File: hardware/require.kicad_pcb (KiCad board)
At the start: 6 copper layers, 70 x 25.4 mm, 99 parts, among them J1 Conn_01x02, U100 SY8089AAC, U1000 RK3308, U15 SY8088AAC, U200 SY8089AAC, U3 EMMC_BGA_153, U300 SY8089AAC, U3000 DDR3_FBGA96, U6000 ap6255, Y1 Crystal_GND24

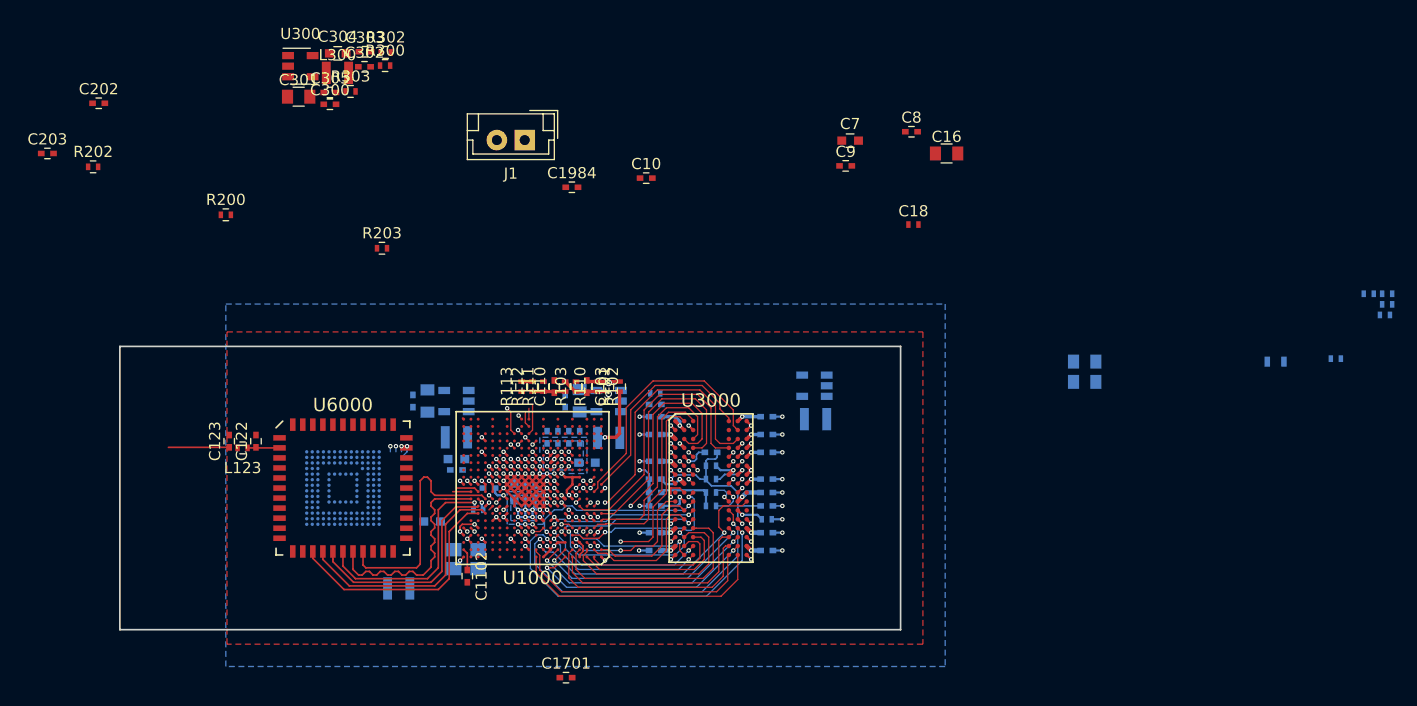
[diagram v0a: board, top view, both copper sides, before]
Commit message: wip
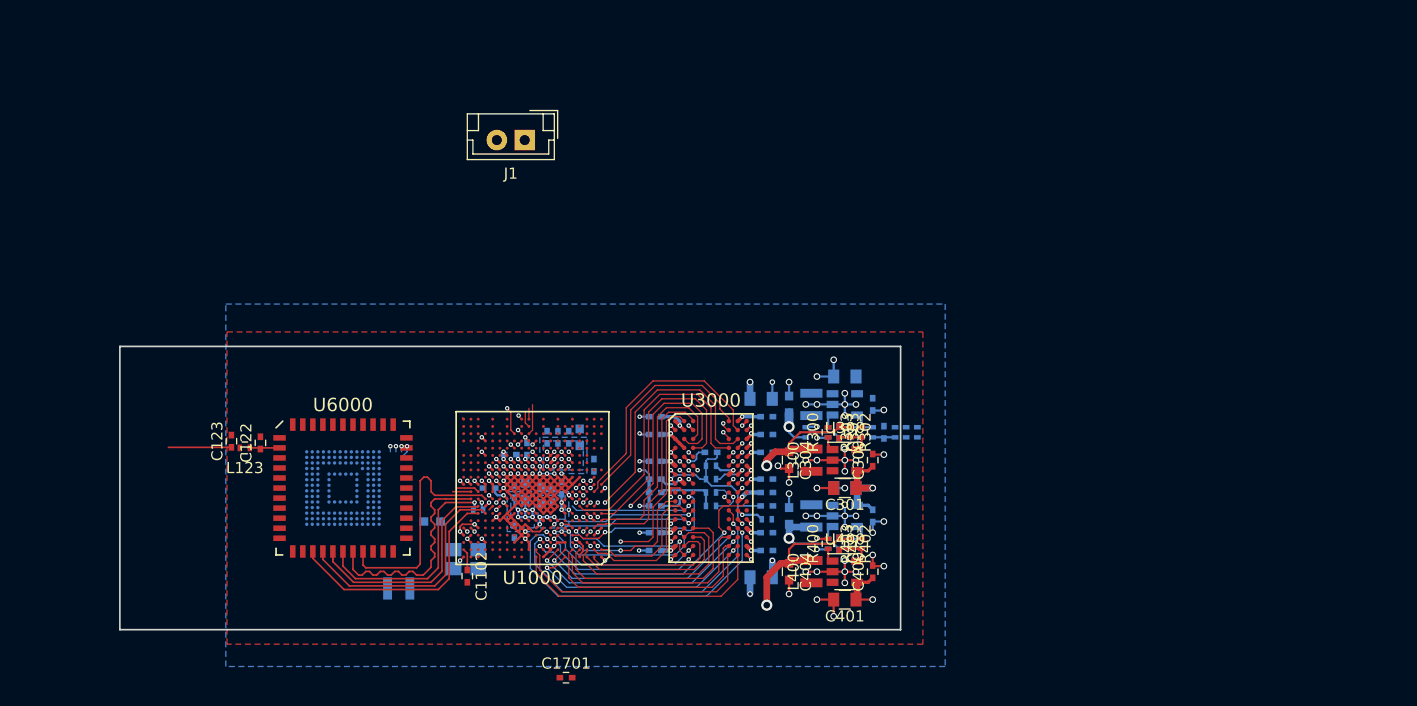
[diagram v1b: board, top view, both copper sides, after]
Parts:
- removed C10: C, Capacitors_SMD:C_0402
- removed C102, C202, C302: 1n, Capacitors_SMD:C_0402
- removed C16: 10uF,10V,X5R, Capacitors_SMD:C_0805
- removed C18: 1u, Resistors_SMD:R_0402_NoSilk
- removed C20: 22p, Resistors_SMD:R_0402_NoSilk
- removed C205, C305: 0.1u, Capacitors_SMD:C_0402
- removed C22: 22u, Resistors_SMD:R_0603
- removed C24: 0.1u, Resistors_SMD:R_0402_NoSilk
- removed L3: 3.3u, require:L_murata_2520
- removed R10: 10, Resistors_SMD:R_0402_NoSilk
- removed R7: 10k, Resistors_SMD:R_0402_NoSilk
- removed R9: 100,5%, Resistors_SMD:R_0402_NoSilk
- removed U15: SY8088AAC, TO_SOT_Packages_SMD:SOT-23-5
- added C400: 0.1u,10V, Capacitors_SMD:C_0402, F.Cu at (95.5, 72.5)
- added C401: 10u,10V, Capacitors_SMD:C_0805, F.Cu at (93.0, 75.0)
- added C403: 22p, Capacitors_SMD:C_0402, F.Cu at (92.5, 70.0)
- added C404: 22u, Capacitors_SMD:C_0603, F.Cu at (88.0, 72.5)
- added C5123: 0.1u, Capacitors_SMD:C_0402, B.Cu at (64.5, 61.5)
- added C5124: 0.1u, Capacitors_SMD:C_0402, B.Cu at (70.5, 63.0)
- added L400: 2.2u, require:L_murata_2520, F.Cu at (90.0, 72.5)
- added R400: 10k, Resistors_SMD:R_0402, F.Cu at (91.5, 70.0)
- added R402: 110k,1%, Resistors_SMD:R_0402, F.Cu at (93.5, 70.0)
- added R403: 150k,1%, Resistors_SMD:R_0402, F.Cu at (94.5, 70.0)
- added U400: SY8089AAC, TO_SOT_Packages_SMD:SOT-23-5, F.Cu at (93.0, 72.5)
- C103, C110, C1984, C203, R101, R102, R103, R110, R111, R112, R113, R200, R202, R203: moved to B.Cu
- C107: value 0.1u -> 2.2u
- C108: value 0.1u -> 22u; footprint Capacitors_SMD:C_0402 -> Capacitors_SMD:C_0603
- C310: renamed from C7; value C -> 10u; moved to B.Cu
- C311: renamed from C8; value C -> 0.1u; moved to B.Cu
- C312: renamed from C9; value C -> 0.1u; moved to B.Cu
- moved C203 79.2 mm to (92.5, 70.0), turned to 90 degrees
- moved R202 75.8 mm to (93.5, 70.0), turned to 90 degrees
- moved R200 61.5 mm to (91.5, 70.0), turned to 270 degrees
- moved U300 60.3 mm to (93.0, 62.5)
- moved C301 60.2 mm to (93.0, 65.0), turned to 180 degrees
- moved C300 58.2 mm to (95.5, 62.5), turned to 90 degrees
- moved R303 55.1 mm to (94.5, 60.0), turned to 90 degrees
- moved L300 54.9 mm to (90.0, 62.5), turned to 90 degrees
- moved C303 54.5 mm to (92.5, 60.0), turned to 270 degrees
- moved C304 54.5 mm to (88.0, 62.5), turned to 270 degrees
- moved R302 53.8 mm to (93.5, 60.0), turned to 270 degrees
- moved R300 51.6 mm to (91.5, 60.0), turned to 90 degrees
- moved R203 50.5 mm to (94.5, 70.0), turned to 270 degrees
- moved C311 45.8 mm to (66.8, 65.7), turned to 90 degrees
- moved C200 42.5 mm to (95.5, 67.5), turned to 270 degrees
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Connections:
- C303 pad 1: VDD_CORE -> VCC_DDR
- C304 pad 1: VDD_CORE -> VCC_DDR
- L300 pad 2: VDD_CORE -> VCC_DDR
- R302 pad 1: VDD_CORE -> VCC_DDR
- U1000 pad G15: Net-(U1000-PadG15) -> GND
- U1000 pad N2: (no net) -> Net-(U1000-PadN2)
- U1000 pad N3: (no net) -> /rk3308-lcdc-mac-i2s1-jtag/WIFI_WAKE_HOST
- U1000 pad N4: (no net) -> Net-(U1000-PadN4)
- U1000 pad N5: (no net) -> VCC_IO
- U1000 pad P3: (no net) -> /rk3308-lcdc-mac-i2s1-jtag/WIFI_REG_ON
- U1000 pad P4: (no net) -> Net-(U1000-PadP4)
- U1000 pad R11: (no net) -> VCC_IO
- U1000 pad R3: (no net) -> Net-(U1000-PadR3)
- U1000 pad R4: (no net) -> Net-(U1000-PadR4)
- U1000 pad R9: (no net) -> Net-(U1000-PadR9)
- U1000 pad T1: (no net) -> Net-(U1000-PadT1)
- U1000 pad T10: (no net) -> /rk3308-lcdc-mac-i2s1-jtag/SPI2_CS
- U1000 pad T2: (no net) -> Net-(U1000-PadT2)
- U1000 pad T3: (no net) -> Net-(U1000-PadT3)
- U1000 pad T4: (no net) -> Net-(U1000-PadT4)
- U1000 pad T5: (no net) -> Net-(U1000-PadT5)
- U1000 pad T6: (no net) -> Net-(U1000-PadT6)
- U1000 pad T8: (no net) -> Net-(U1000-PadT8)
- U1000 pad T9: (no net) -> /rk3308-lcdc-mac-i2s1-jtag/SPI2_TX_UART2_TX_M0
- U1000 pad U2: (no net) -> Net-(U1000-PadU2)
- U1000 pad U3: (no net) -> Net-(U1000-PadU3)
- U1000 pad U4: (no net) -> Net-(U1000-PadU4)
- U1000 pad U5: (no net) -> Net-(U1000-PadU5)
- U1000 pad U6: (no net) -> Net-(U1000-PadU6)
- U1000 pad U7: (no net) -> Net-(U1000-PadU7)
- U1000 pad U8: (no net) -> Net-(U1000-PadU8)
- U1000 pad U9: (no net) -> Net-(U1000-PadU9)
- U1000 pad V1: (no net) -> Net-(U1000-PadV1)
- U1000 pad V10: (no net) -> /rk3308-lcdc-mac-i2s1-jtag/SPI2_CLK
- U1000 pad V2: (no net) -> Net-(U1000-PadV2)
- U1000 pad V3: (no net) -> Net-(U1000-PadV3)
- U1000 pad V4: (no net) -> Net-(U1000-PadV4)
- U1000 pad V5: (no net) -> Net-(U1000-PadV5)
- U1000 pad V6: (no net) -> Net-(U1000-PadV6)
- U1000 pad V7: (no net) -> Net-(U1000-PadV7)
- U1000 pad V8: (no net) -> Net-(U1000-PadV8)
- U1000 pad V9: (no net) -> Net-(U1000-PadV9)
- U1000 pad W1: (no net) -> Net-(U1000-PadW1)
- U1000 pad W2: (no net) -> Net-(U1000-PadW2)
- U1000 pad W3: (no net) -> Net-(U1000-PadW3)
- U1000 pad W4: (no net) -> Net-(U1000-PadW4)
- U1000 pad W5: (no net) -> Net-(U1000-PadW5)
- U1000 pad W6: (no net) -> Net-(U1000-PadW6)
- U1000 pad W7: (no net) -> Net-(U1000-PadW7)
- U1000 pad W9: (no net) -> /rk3308-lcdc-mac-i2s1-jtag/SPI2_RX_UART2_RX_M0
- U1000 pad Y2: (no net) -> Net-(U1000-PadY2)
- U1000 pad Y3: (no net) -> Net-(U1000-PadY3)
- U1000 pad Y5: (no net) -> Net-(U1000-PadY5)
- U1000 pad Y7: (no net) -> Net-(U1000-PadY7)
- U1000 pad Y9: (no net) -> Net-(U1000-PadY9)
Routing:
- net GND: track 125.6 -> 195.7 mm, vias 109 -> 126
- net VCC_DDR: track 32.8 -> 52.3 mm, vias 23 -> 25
- net VCC5V0_SYS: track 1.84 -> 17.0 mm, vias 0 -> 5
- net VCC_IO: track 0.00 -> 14.4 mm, vias 0 -> 1
- net VDD_CORE: track 24.7 -> 38.1 mm
- net VDD_LOG: track 10.6 -> 19.0 mm, vias 6 -> 7
- net /ddr/DDR_CASN: track 16.0 -> 11.9 mm
- net Net-(C403-Pad2): track 0.00 -> 3.54 mm
- net Net-(C203-Pad2): track 0.00 -> 3.51 mm
- net Net-(C303-Pad2): track 0.00 -> 3.31 mm
- net Net-(R400-Pad1): track 0.00 -> 1.50 mm
- net Net-(R200-Pad1): track 0.00 -> 1.47 mm
- net /ddr/DDR_DQS0N: track 0.00 -> 1.33 mm, vias 0 -> 2
- net /ddr/DDR_DQS0P: track 0.00 -> 1.27 mm, vias 0 -> 2
- net Net-(R300-Pad1): track 0.00 -> 1.27 mm
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- added copper zone on In4.Cu, net VCC5V0_SYS
- added copper zone on B.Cu, net VCC_DDR
- added copper zone on In3.Cu, net VDD_LOG
